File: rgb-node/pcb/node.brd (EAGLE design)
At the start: 54 x 17 mm, 19 parts, among them U2 MCP1640

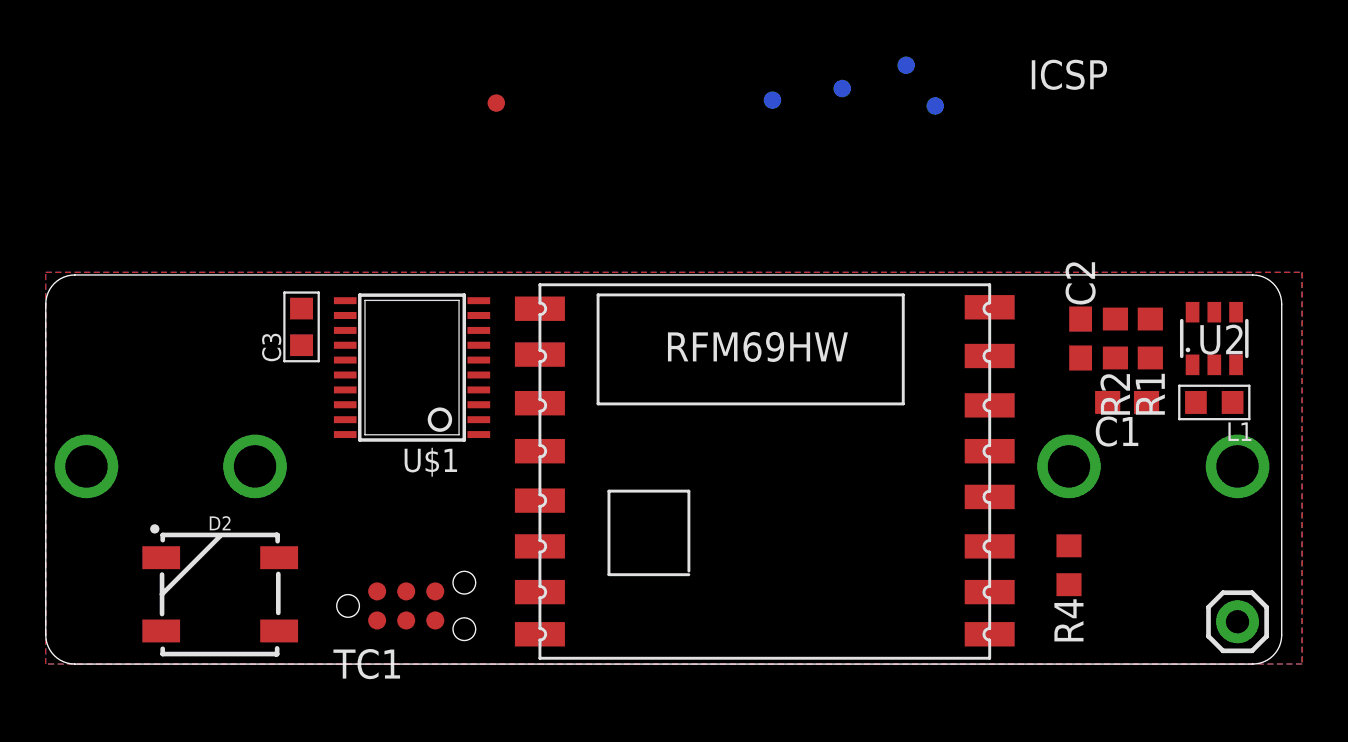
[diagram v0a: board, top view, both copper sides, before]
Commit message: dumped some things on the pcb
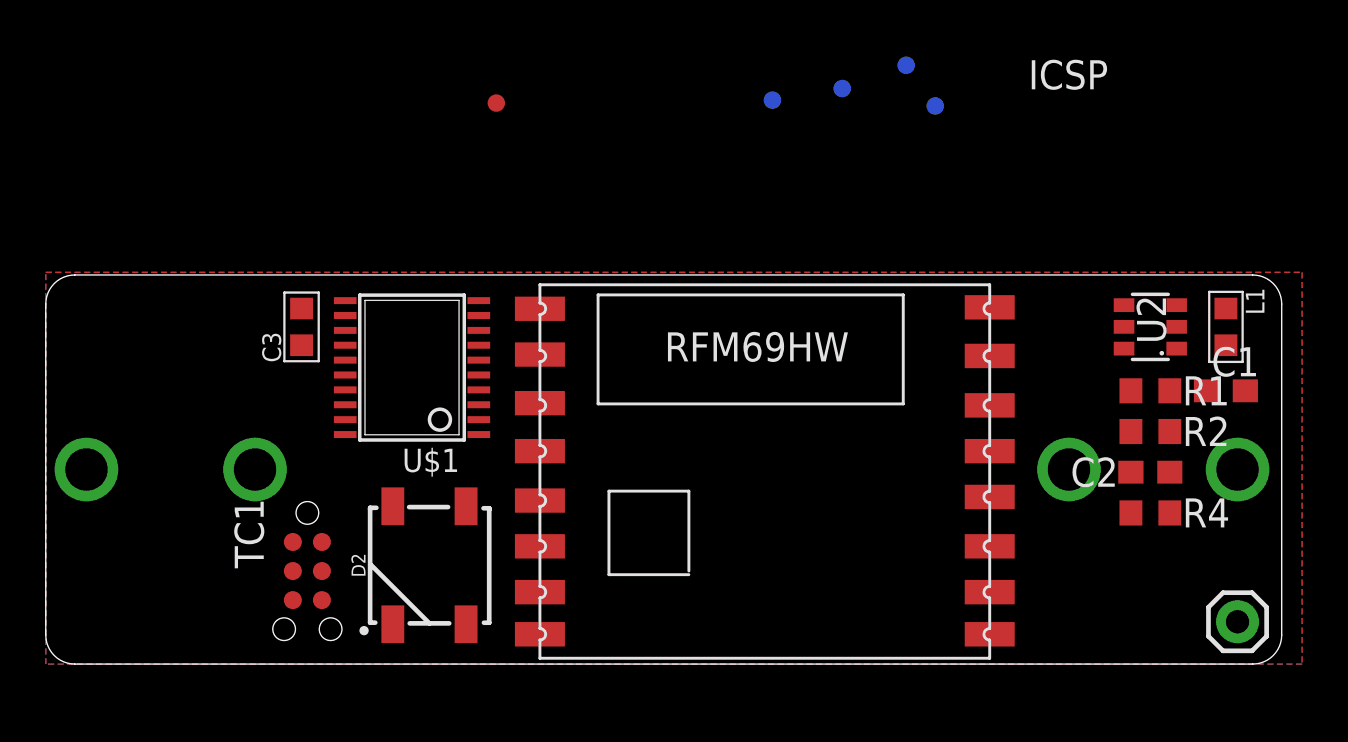
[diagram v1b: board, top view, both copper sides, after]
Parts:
- moved D2 9.23 mm to (16.8, 4.32), turned to 90 degrees
- moved C2 6.59 mm to (48.3, 8.38), turned to 0 degrees
- moved TC1 4.58 mm to (11.4, 4.06), turned to 270 degrees
- moved C1 4.35 mm to (51.6, 11.9), turned to 0 degrees
- moved R2 4.34 mm to (48.3, 10.2), turned to 0 degrees
- moved R4 4.23 mm to (48.3, 6.60), turned to 180 degrees
- moved L1 3.34 mm to (51.6, 14.7), turned to 270 degrees
- moved U2 2.84 mm to (48.3, 14.7), turned to 90 degrees
- moved R1 2.29 mm to (48.3, 11.9), turned to 0 degrees
- moved BAT2 0.14 mm to (26.9, 8.50)
